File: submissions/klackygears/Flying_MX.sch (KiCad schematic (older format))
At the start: 37 parts, among them J1 USB_C_Receptacle, SW1 SW_Push, U1 ATmega32U4-AU, U2 PRTR5V0U2X, Y1 16MHz

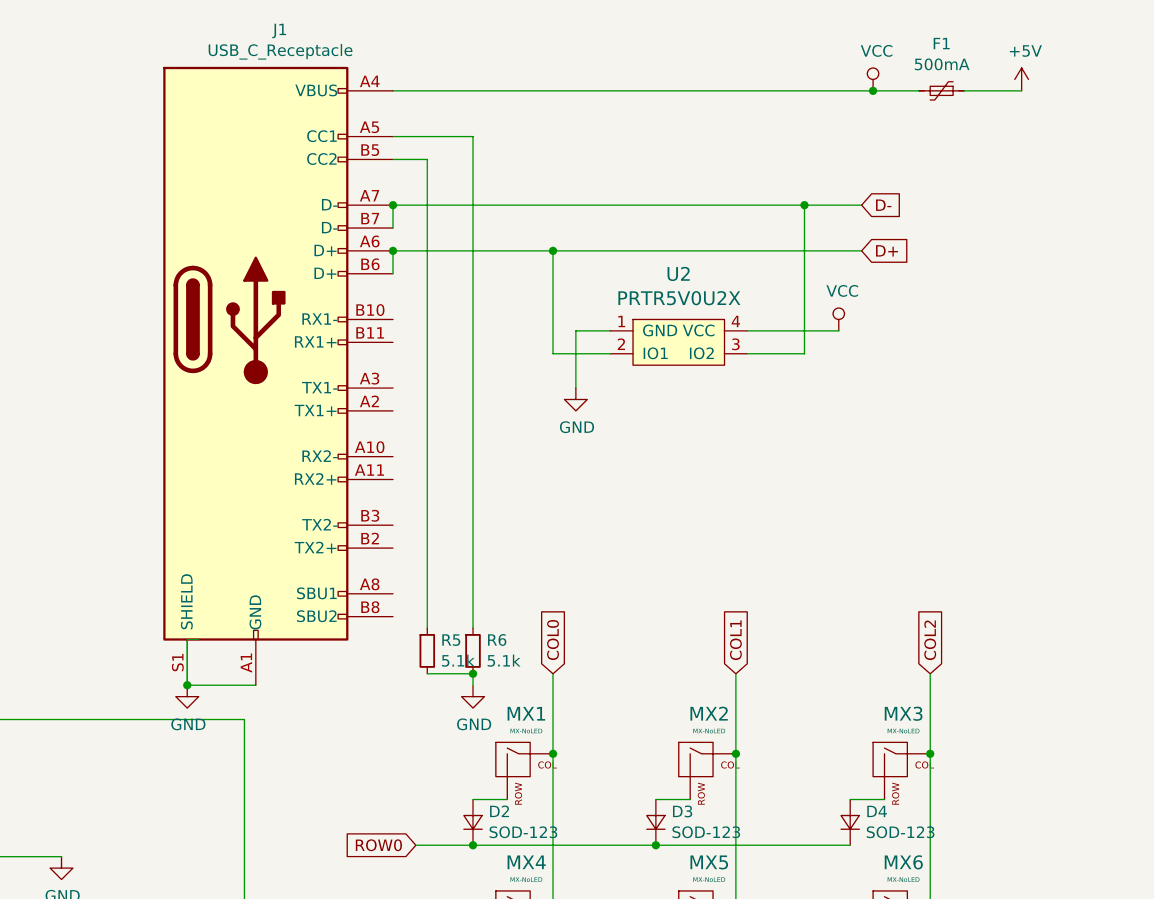
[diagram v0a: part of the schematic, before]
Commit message: correcting & improving some things
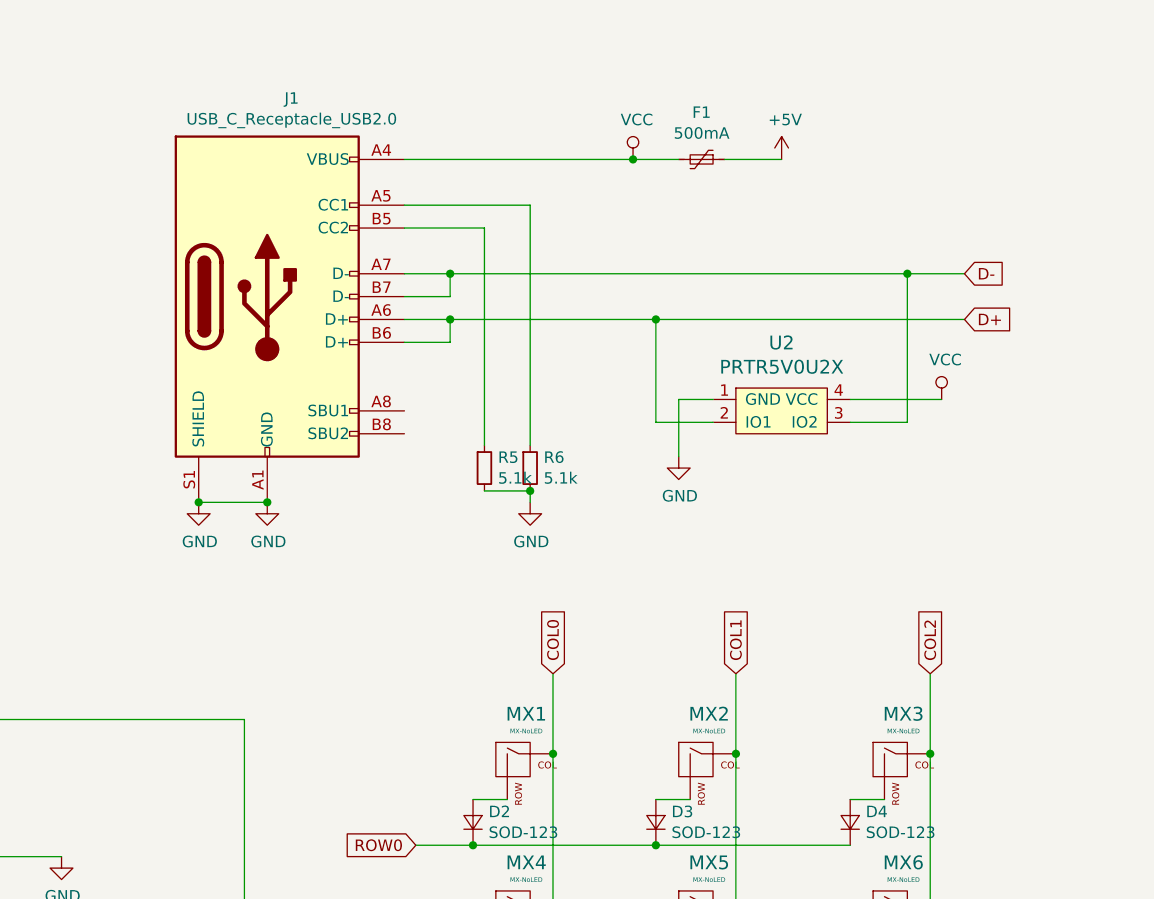
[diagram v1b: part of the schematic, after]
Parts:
- removed J1: USB_C_Receptacle, Connector_USB:USB_C_Receptacle_GCT_USB4085, symbol Connector:USB_C_Receptacle
- added J1: USB_C_Receptacle_USB2.0, Connector_USB:USB_C_Receptacle_GCT_USB4085, symbol Connector:USB_C_Receptacle_USB2.0
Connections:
- net D+: now also J1.A6 (D+), J1.B6 (D+)
- net D-: now also J1.A7 (D-), J1.B7 (D-)
- net GND: now also J1.A1 (GND), J1.A12 (GND), J1.B1 (GND), J1.B12 (GND), J1.S1 (SHIELD)
- net VCC: now also J1.A4 (VBUS), J1.A9 (VBUS), J1.B4 (VBUS), J1.B9 (VBUS)
- net at R5.1: now also J1.B5 (CC2)
- net at R6.1: now also J1.A5 (CC1)

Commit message: updating footprints and silk
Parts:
- D10, D11, D12, D13, D8, D9: footprint KiCadLibs:SK6812MINI-E -> Flying_MX:SK6812MINI-E
- MX1, MX2, MX3, MX4, MX5, MX6: footprint Universal-Switch-Footprint:MX-ALPs-PG1350-FLIP -> Flying_MX:MX-ALPs-PG1350-FLIP; symbol MX_Alps_Hybrid:MX-NoLED -> Flying_MX:MX-NoLED
- SW1: footprint random-keyboard-parts:SKQG-1155865 -> Flying_MX:SKQG-1155865
- U2: footprint random-keyboard-parts:SOT143B -> Flying_MX:SOT143B; symbol random-keyboard-parts:PRTR5V0U2X -> Flying_MX:PRTR5V0U2X
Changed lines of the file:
@@
 F 0 "D13" H 8944 6046 50  0000 L CNN
 F 1 "SK6812MINI" H 8944 5955 50  0000 L CNN
-F 2 "KiCadLibs:SK6812MINI-E" H 8650 5700 50  0001 L TNN
+F 2 "Flying_MX:SK6812MINI-E" H 8650 5700 50  0001 L TNN
 F 3 "https://cdn-shop.adafruit.com/product-files/2686/SK6812MINI_REV.01-1-2.pdf" H 8700 5625 50  0001 L TNN
 	1    8600 6000
@@
 F 0 "D12" H 7894 6046 50  0000 L CNN
 F 1 "SK6812MINI" H 7894 5955 50  0000 L CNN
-F 2 "KiCadLibs:SK6812MINI-E" H 7600 5700 50  0001 L TNN
+F 2 "Flying_MX:SK6812MINI-E" H 7600 5700 50  0001 L TNN
 F 3 "https://cdn-shop.adafruit.com/product-files/2686/SK6812MINI_REV.01-1-2.pdf" H 7650 5625 50  0001 L TNN
 	1    7550 6000
@@
 F 0 "D11" H 6844 6046 50  0000 L CNN
 F 1 "SK6812MINI" H 6844 5955 50  0000 L CNN
-F 2 "KiCadLibs:SK6812MINI-E" H 6550 5700 50  0001 L TNN
+F 2 "Flying_MX:SK6812MINI-E" H 6550 5700 50  0001 L TNN
 F 3 "https://cdn-shop.adafruit.com/product-files/2686/SK6812MINI_REV.01-1-2.pdf" H 6600 5625 50  0001 L TNN
 	1    6500 6000
@@
 F 0 "D10" H 8944 5246 50  0000 L CNN
 F 1 "SK6812MINI" H 8944 5155 50  0000 L CNN
-F 2 "KiCadLibs:SK6812MINI-E" H 8650 4900 50  0001 L TNN
+F 2 "Flying_MX:SK6812MINI-E" H 8650 4900 50  0001 L TNN
 F 3 "https://cdn-shop.adafruit.com/product-files/2686/SK6812MINI_REV.01-1-2.pdf" H 8700 4825 50  0001 L TNN
 	1    8600 5200
@@
 F 0 "D9" H 7894 5246 50  0000 L CNN
 F 1 "SK6812MINI" H 7894 5155 50  0000 L CNN
-F 2 "KiCadLibs:SK6812MINI-E" H 7600 4900 50  0001 L TNN
+F 2 "Flying_MX:SK6812MINI-E" H 7600 4900 50  0001 L TNN
 F 3 "https://cdn-shop.adafruit.com/product-files/2686/SK6812MINI_REV.01-1-2.pdf" H 7650 4825 50  0001 L TNN
 	1    7550 5200
@@
 F 0 "D8" H 6844 5246 50  0000 L CNN
 F 1 "SK6812MINI" H 6844 5155 50  0000 L CNN
-F 2 "KiCadLibs:SK6812MINI-E" H 6550 4900 50  0001 L TNN
+F 2 "Flying_MX:SK6812MINI-E" H 6550 4900 50  0001 L TNN
 F 3 "https://cdn-shop.adafruit.com/product-files/2686/SK6812MINI_REV.01-1-2.pdf" H 6600 4825 50  0001 L TNN
 	1    6500 5200
@@
 $EndComp
 $Comp
-L MX_Alps_Hybrid:MX-NoLED MX6
+L Flying_MX:MX-NoLED MX6
 U 1 1 5E948146
 P 8650 4250
 F 0 "MX6" H 8683 4473 60  0000 C CNN
 F 1 "MX-NoLED" H 8683 4399 20  0000 C CNN
-F 2 "Universal-Switch-Footprint:MX-ALPs-PG1350-FLIP" H 8025 4225 60  0001 C CNN
+F 2 "Flying_MX:MX-ALPs-PG1350-FLIP" H 8025 4225 60  0001 C CNN
 F 3 "" H 8025 4225 60  0001 C CNN
 	1    8650 4250
@@
 $EndComp
 $Comp
-L MX_Alps_Hybrid:MX-NoLED MX3
+L Flying_MX:MX-NoLED MX3
 U 1 1 5E947AB0
 P 8650 3600
 F 0 "MX3" H 8683 3823 60  0000 C CNN
 F 1 "MX-NoLED" H 8683 3749 20  0000 C CNN
-F 2 "Universal-Switch-Footprint:MX-ALPs-PG1350-FLIP" H 8025 3575 60  0001 C CNN
+F 2 "Flying_MX:MX-ALPs-PG1350-FLIP" H 8025 3575 60  0001 C CNN
 F 3 "" H 8025 3575 60  0001 C CNN
 	1    8650 3600
@@
 $EndComp
 $Comp
-L MX_Alps_Hybrid:MX-NoLED MX5
+L Flying_MX:MX-NoLED MX5
 U 1 1 5E94745B
 P 7800 4250
 F 0 "MX5" H 7833 4473 60  0000 C CNN
 F 1 "MX-NoLED" H 7833 4399 20  0000 C CNN
-F 2 "Universal-Switch-Footprint:MX-ALPs-PG1350-FLIP" H 7175 4225 60  0001 C CNN
+F 2 "Flying_MX:MX-ALPs-PG1350-FLIP" H 7175 4225 60  0001 C CNN
 F 3 "" H 7175 4225 60  0001 C CNN
 	1    7800 4250
@@
 $EndComp
 $Comp
-L MX_Alps_Hybrid:MX-NoLED MX4
+L Flying_MX:MX-NoLED MX4
 U 1 1 5E946C3A
 P 7000 4250
 F 0 "MX4" H 7033 4473 60  0000 C CNN
 F 1 "MX-NoLED" H 7033 4399 20  0000 C CNN
-F 2 "Universal-Switch-Footprint:MX-ALPs-PG1350-FLIP" H 6375 4225 60  0001 C CNN
+F 2 "Flying_MX:MX-ALPs-PG1350-FLIP" H 6375 4225 60  0001 C CNN
 F 3 "" H 6375 4225 60  0001 C CNN
 	1    7000 4250
@@
 $EndComp
 $Comp
-L MX_Alps_Hybrid:MX-NoLED MX2
+L Flying_MX:MX-NoLED MX2
 U 1 1 5E945CA6
 P 7800 3600
 F 0 "MX2" H 7833 3823 60  0000 C CNN
 F 1 "MX-NoLED" H 7833 3749 20  0000 C CNN
-F 2 "Universal-Switch-Footprint:MX-ALPs-PG1350-FLIP" H 7175 3575 60  0001 C CNN
+F 2 "Flying_MX:MX-ALPs-PG1350-FLIP" H 7175 3575 60  0001 C CNN
 F 3 "" H 7175 3575 60  0001 C CNN
 	1    7800 3600
@@
 $EndComp
 $Comp
-L MX_Alps_Hybrid:MX-NoLED MX1
+L Flying_MX:MX-NoLED MX1
 U 1 1 5E94506F
 P 7000 3600
 F 0 "MX1" H 7033 3823 60  0000 C CNN
 F 1 "MX-NoLED" H 7033 3749 20  0000 C CNN
-F 2 "Universal-Switch-Footprint:MX-ALPs-PG1350-FLIP" H 6375 3575 60  0001 C CNN
+F 2 "Flying_MX:MX-ALPs-PG1350-FLIP" H 6375 3575 60  0001 C CNN
 F 3 "" H 6375 3575 60  0001 C CNN
 	1    7000 3600
@@
 F 0 "SW1" H 2450 2185 50  0000 C CNN
 F 1 "SW_Push" H 2450 2094 50  0000 C CNN
-F 2 "random-keyboard-parts:SKQG-1155865" H 2450 2100 50  0001 C CNN
+F 2 "Flying_MX:SKQG-1155865" H 2450 2100 50  0001 C CNN
 F 3 "~" H 2450 2100 50  0001 C CNN
 	1    2450 1900
@@
 	8450 2100 8700 2100
 $Comp
-L random-keyboard-parts:PRTR5V0U2X U2
+L Flying_MX:PRTR5V0U2X U2
 U 1 1 5EC5DC49
 P 8150 2050
 F 0 "U2" H 8150 2347 60  0000 C CNN
 F 1 "PRTR5V0U2X" H 8150 2241 60  0000 C CNN
-F 2 "random-keyboard-parts:SOT143B" H 8150 2050 60  0001 C CNN
+F 2 "Flying_MX:SOT143B" H 8150 2050 60  0001 C CNN
 F 3 "" H 8150 2050 60  0001 C CNN
 	1    8150 2050
